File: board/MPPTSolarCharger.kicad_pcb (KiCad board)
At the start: 2 copper layers, 150.5 x 49.5 mm, 49 parts, among them J1 Screw_Terminal_01x02, J2 Screw_Terminal_01x02, J3 Conn_01x06, Q1 PSMN5R5-60YS, Q2 PSMN5R5-60YS, Q3 PSMN5R5-60YS, U1 LM350_TO220, U2 MIC4605-1YM, U3 INA260, U4 INA260

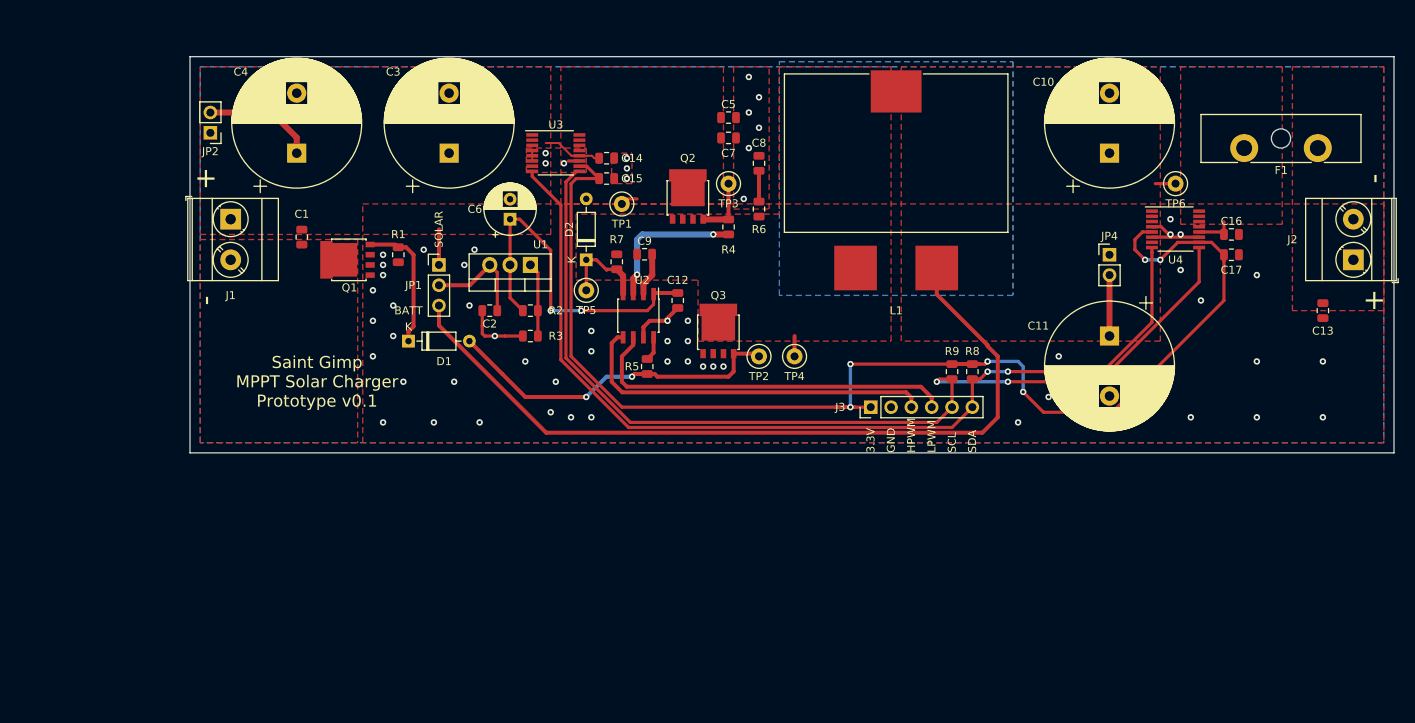
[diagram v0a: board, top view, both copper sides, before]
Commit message: Rev 2 of board layout, WIP
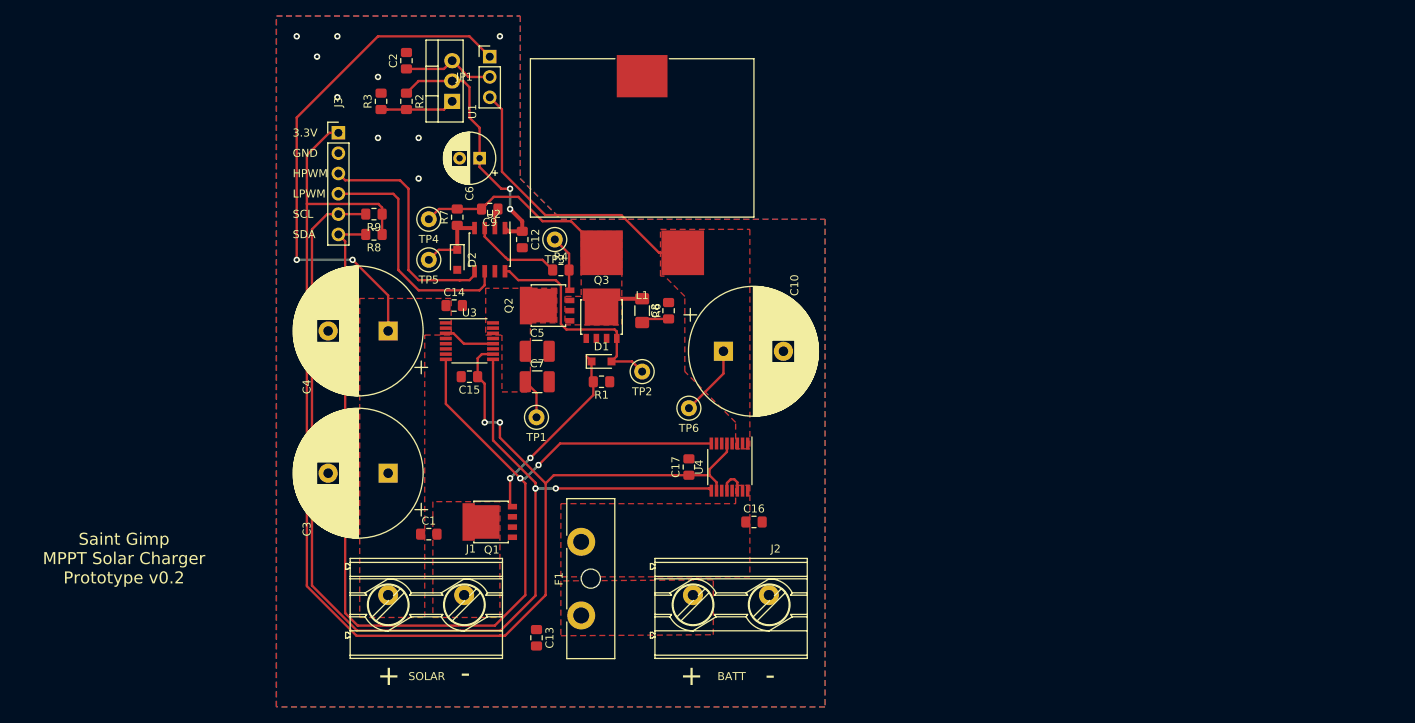
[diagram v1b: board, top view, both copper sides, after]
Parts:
- removed C11: 1000uF, Capacitor_THT:CP_Radial_D16.0mm_P7.50mm
- removed JP2, JP4: Jumper_NC_Small, Connector_PinHeader_2.54mm:PinHeader_1x02_P2.54mm_Vertical
- removed R5: 3.3, Resistor_SMD:R_0805_2012Metric
- C1, C12, C13, C14, C15, C16, C17, C2, C8, C9: footprint Capacitor_SMD:C_0805_2012Metric -> Capacitor_SMD:C_0805_2012Metric_Pad1.15x1.40mm_HandSolder
- C5, C7: footprint Capacitor_SMD:C_0805_2012Metric -> Capacitor_SMD:C_1210_3225Metric_Pad1.42x2.65mm_HandSolder
- D1, D2: footprint Diode_THT:D_DO-35_SOD27_P7.62mm_Horizontal -> Diode_SMD:D_SOD-323_HandSoldering
- J1, J2: footprint TerminalBlock_Phoenix:TerminalBlock_Phoenix_MKDS-3-2-5.08_1x02_P5.08mm_Horizontal -> Saintgimp:Phoenix_Contact_MKDS_5-2-952
- R1, R2, R3, R4, R7, R8, R9: footprint Resistor_SMD:R_0805_2012Metric -> Resistor_SMD:R_0805_2012Metric_Pad1.15x1.40mm_HandSolder
- R6: footprint Resistor_SMD:R_0805_2012Metric -> Resistor_SMD:R_1206_3216Metric_Pad1.42x1.75mm_HandSolder
- moved F1 109.0 mm to (124.5, 143.5), turned to 90 degrees
- moved C13 106.5 mm to (118.9, 146.3)
- moved J2 92.6 mm to (138.4, 141.0), turned to 0 degrees
- moved R8 76.7 mm to (98.6, 95.9), turned to 180 degrees
- moved R9 74.9 mm to (98.6, 93.3), turned to 180 degrees
- moved J3 74.9 mm to (94.1, 83.2), turned to 0 degrees
- moved C17 72.8 mm to (137.9, 125.0), turned to 90 degrees
- moved C16 69.7 mm to (146.1, 131.8)
- moved TP6 67.0 mm to (137.9, 117.6)
- moved U4 63.2 mm to (143.0, 125.0), turned to 270 degrees
- moved C10 54.2 mm to (142.2, 110.5), turned to 0 degrees
- moved J1 50.9 mm to (100.3, 141.0), turned to 0 degrees
- moved TP4 48.8 mm to (105.4, 94.0)
- moved C3 40.7 mm to (100.3, 125.7), turned to 180 degrees
- moved C1 40.4 mm to (105.4, 133.3), turned to 0 degrees
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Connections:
- C4 pad 1: Net-(C4-Pad1) -> /PowerStage/SOLAR+
- C9 pad 1: /PowerStage/SWITCH_NODE -> /PowerStage/HB
- C9 pad 2: /PowerStage/HB -> /PowerStage/SWITCH_NODE
- D1 pad 2: Net-(D1-Pad2) -> /PowerStage/LOW_DRIVER
- Q3 pad 4: Net-(D1-Pad2) -> /PowerStage/LOW_DRIVER
- TP2 pad 1: Net-(D1-Pad2) -> /PowerStage/LOW_DRIVER
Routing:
- net /PowerStage/SOLAR+: track 11.9 -> 71.3 mm, vias 0 -> 2
- net /PowerStage/BUCK_OUT: track 103.0 -> 45.6 mm
- net Net-(D1-Pad2): track 43.1 -> 0.00 mm, vias 2 -> 0
- net /PowerStage/SWITCH_NODE: track 2.54 -> 36.1 mm
- net GND: track 26.1 -> 0.00 mm, vias 60 -> 9
- net /PowerStage/LOW_DRIVER: track 3.04 -> 28.3 mm
- net /MCU/HIGH_PWM: track 46.0 -> 29.4 mm
- net /MCU/LOW_PWM: track 46.9 -> 30.5 mm
- net /MCU/SDA: track 119.3 -> 135.1 mm
- net Net-(C4-Pad1): track 14.0 -> 0.00 mm
- net /MCU/SCL: track 124.4 -> 138.0 mm
- net +10V: track 43.9 -> 32.5 mm
- net +3V3: track 159.8 -> 171.0 mm, vias 6 -> 2
- net Net-(C11-Pad1): track 7.62 -> 0.00 mm
- net /PowerStage/HIGH_DRIVER: track 18.7 -> 11.3 mm, vias 2 -> 0
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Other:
- board outline removed
- board text added: "Saint Gimp MPPT Solar Charger Prototype v0.2"
- board text removed: "Saint Gimp MPPT Solar Charger Prototype v0.1"
